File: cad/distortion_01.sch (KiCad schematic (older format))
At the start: 90 parts

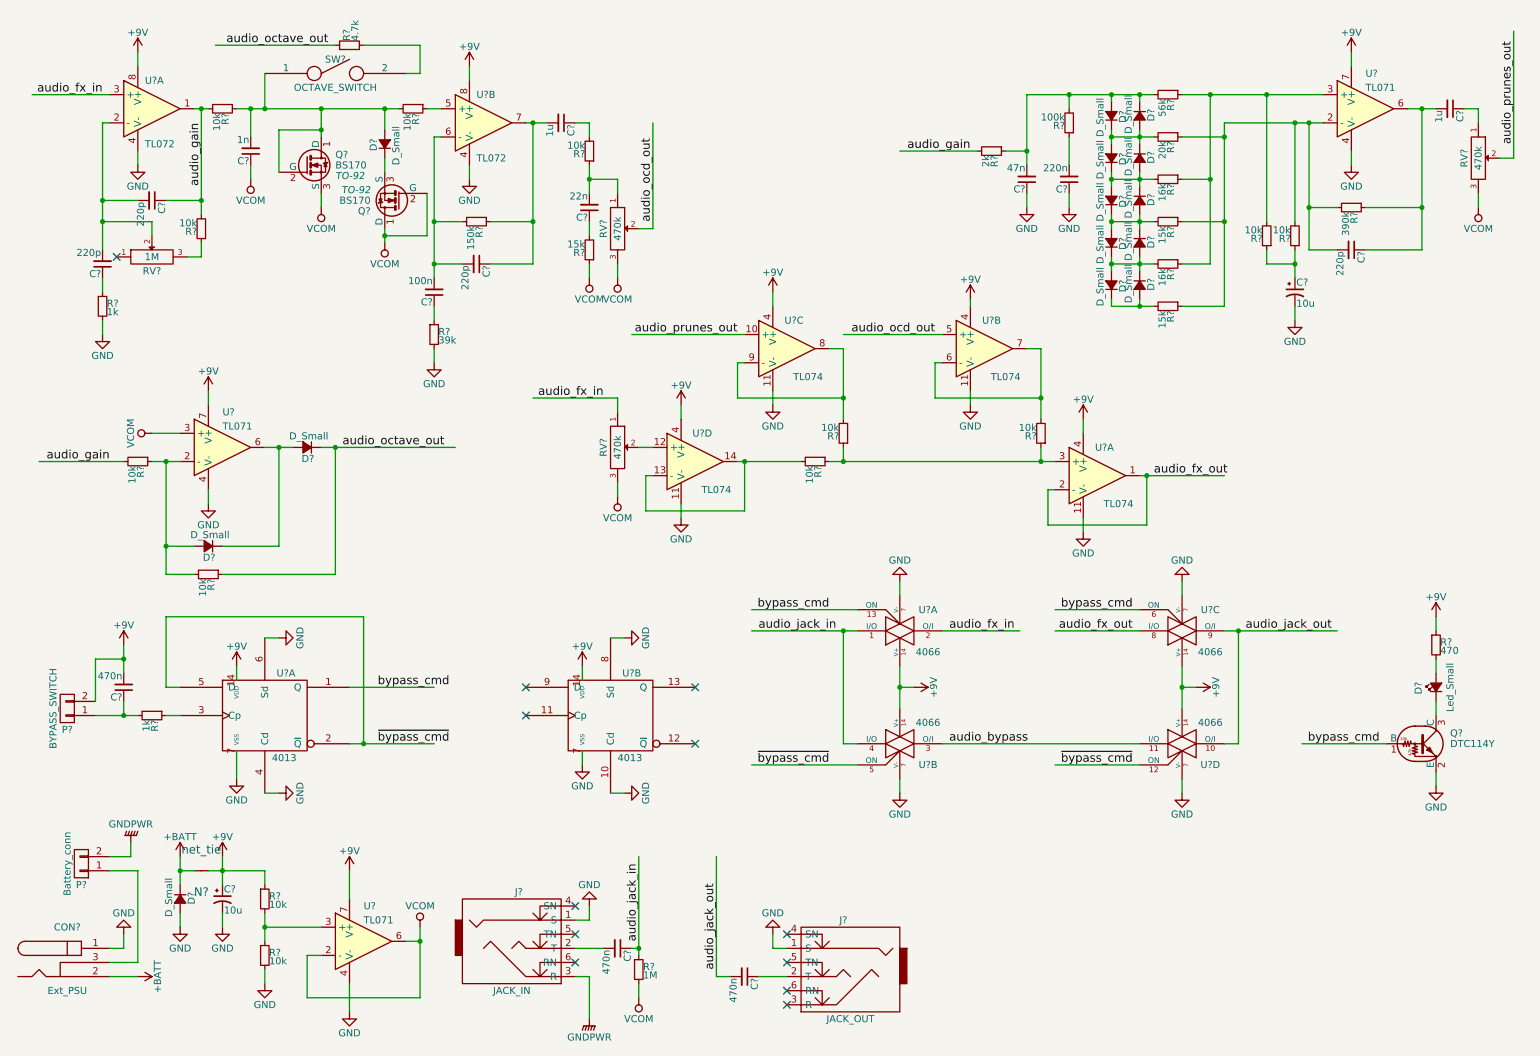
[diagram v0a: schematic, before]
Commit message: Simulated OCD / octave part.
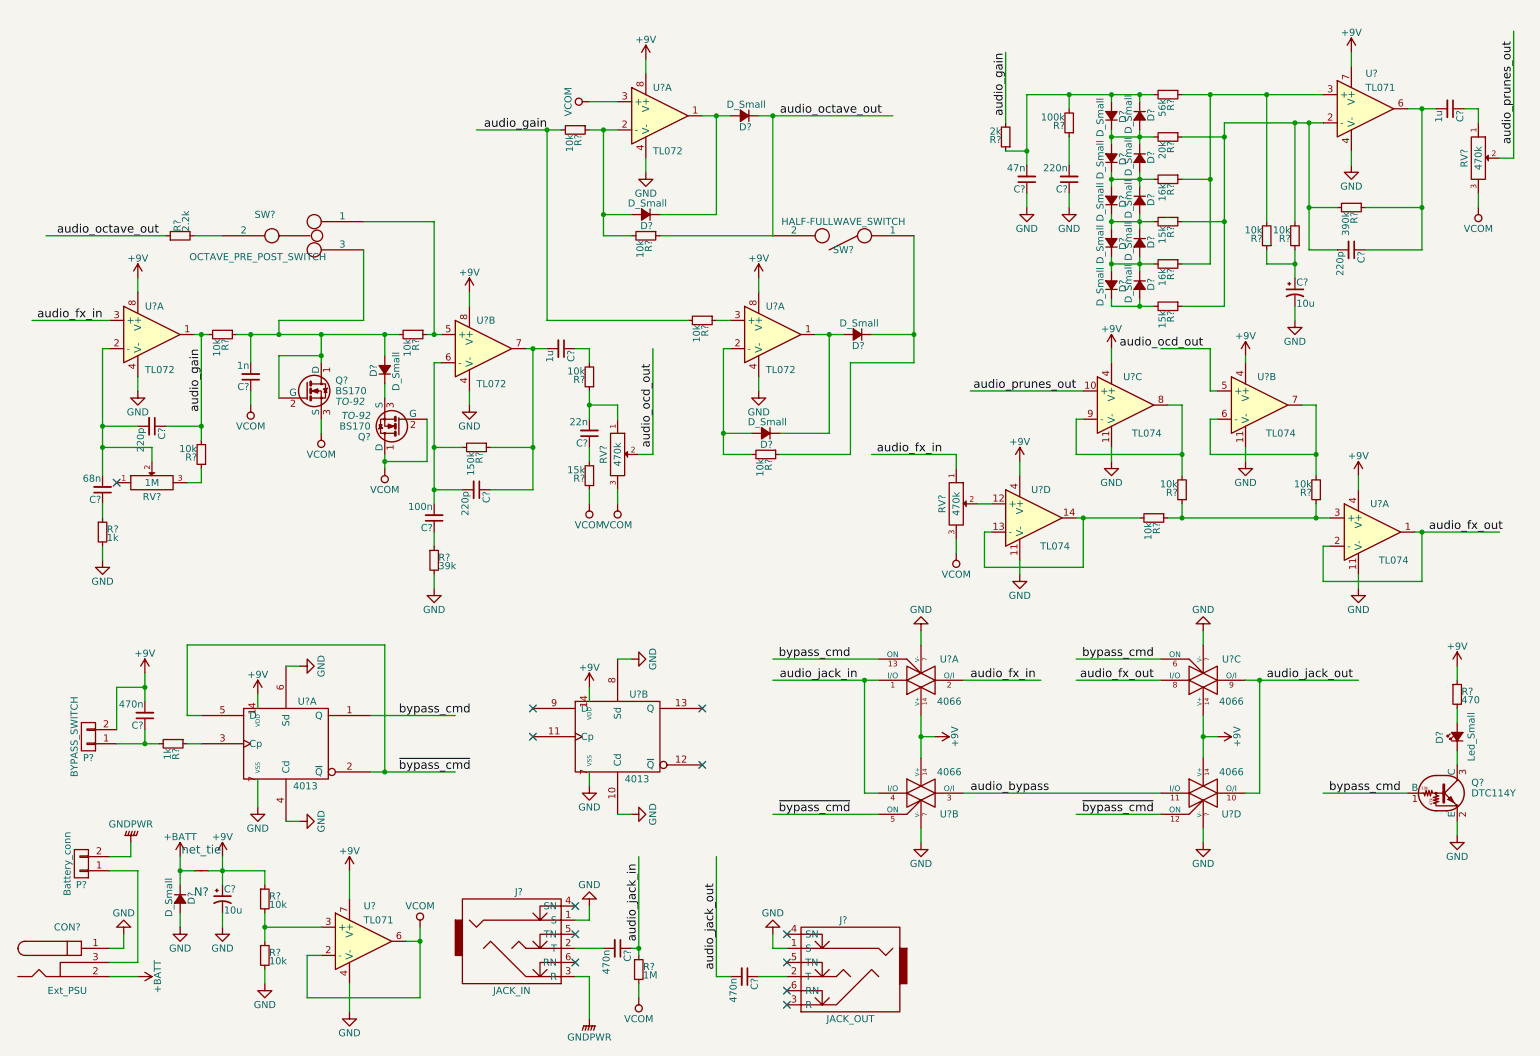
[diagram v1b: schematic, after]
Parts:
- removed SW?: OCTAVE_SWITCH, symbol SPST
- removed U?: TL071, symbol TL071
- added D? (x2): D_Small, symbol D_Small
- added R? (x2): 10k, symbol R_Small
- added SW?: OCTAVE_PRE_POST_SWITCH, symbol SWITCH_INV_MSM
- added SW?: HALF-FULLWAVE_SWITCH, symbol SPST
- added U? (x2): TL072, symbol TL072
- C?: value 220p -> 68n
- R?: value 4.7k -> 2.2k
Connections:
- wire segments 244 -> 265
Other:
- moved on the sheet: C?, D?, P?, Q?, R?, RV?, U?A, U?B, U?C, U?D
